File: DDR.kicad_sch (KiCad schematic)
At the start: 30 parts

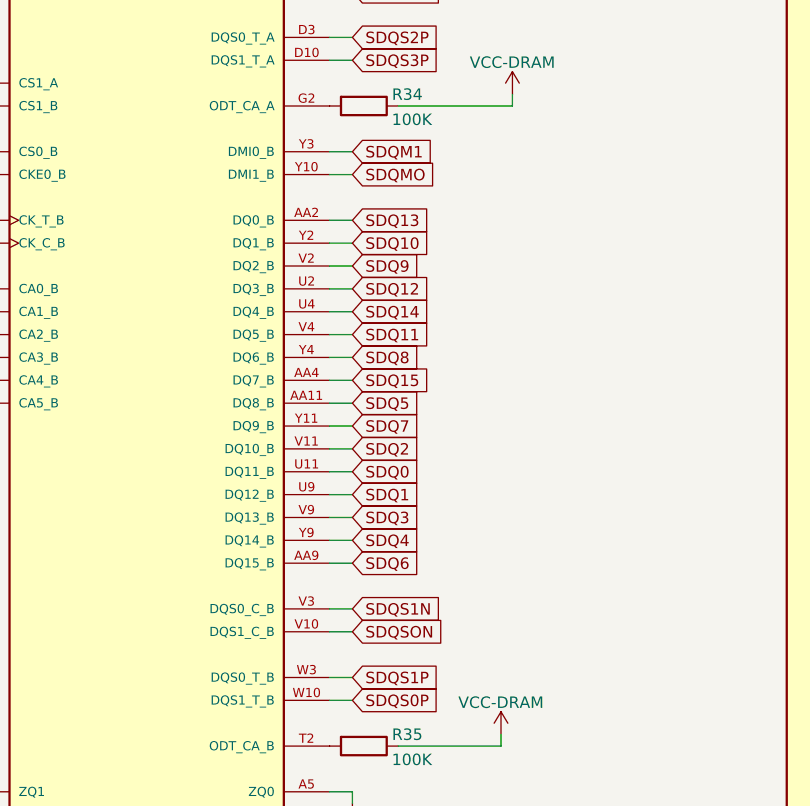
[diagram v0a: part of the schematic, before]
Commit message: Пытаюсь сделать трассировку DDК
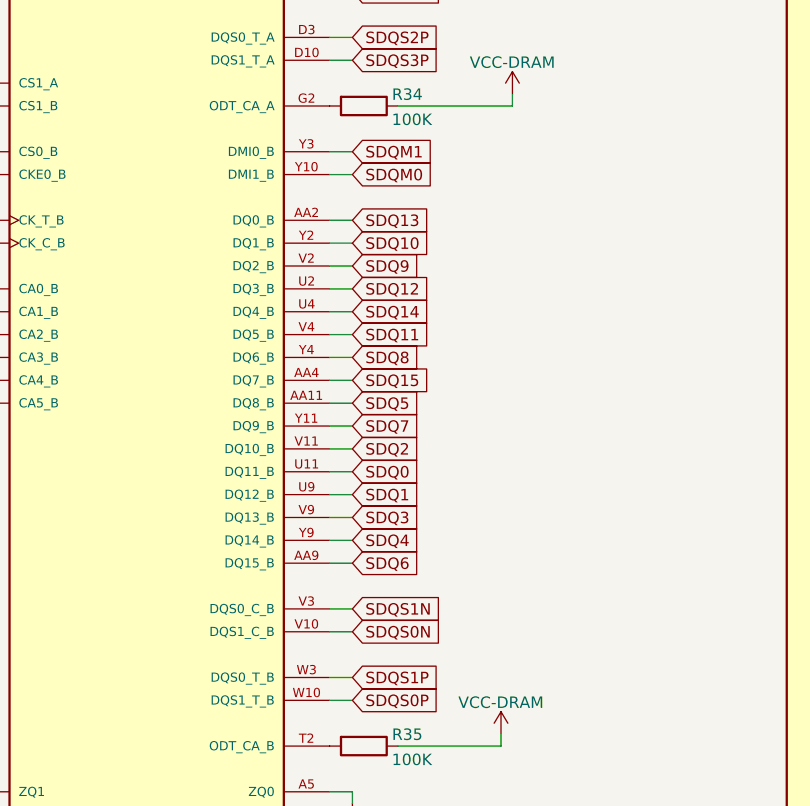
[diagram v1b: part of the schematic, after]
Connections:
- net SDQMO renamed SDQM0
- net SDQSON renamed SDQS0N
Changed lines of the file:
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@@
 	(wire
 		(pts
-			(xy 109.22 143.51) (xy 106.68 143.51)
-		)
-		(stroke
-			(width 0)
-			(type default)
-		)
-	)
-	(wire
-		(pts
 			(xy 288.29 130.81) (xy 302.26 130.81)
 		)
@@
 	(wire
 		(pts
+			(xy 109.22 143.51) (xy 106.68 143.51)
+		)
+		(stroke
+			(width 0)
+			(type default)
+		)
+	)
+	(wire
+		(pts
 			(xy 135.89 236.22) (xy 142.24 236.22)
 		)
@@
 		)
 	)
-	(global_label "SDQMO"
+	(global_label "SDQM0"
 		(shape input)
 		(at 152.4 130.81 0)
@@
 		)
 	)
-	(global_label "SDQSON"
+	(global_label "SDQS0N"
 		(shape input)
 		(at 152.4 181.61 0)
@@
 		)
 		(property "Intersheetrefs" "${INTERSHEET_REFS}"
-			(at 161.8561 181.61 0)
+			(at 162.9447 181.61 0)
 			(effects
 				(font
